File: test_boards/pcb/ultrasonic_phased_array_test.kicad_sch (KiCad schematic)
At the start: 18 parts, among them J1 DF40C-80DP-0.4V, U1 OPA2626, U2 OPA2626, U3 OPA2626, U43 AD7699BCP, U45 SN74LV1T34DBV

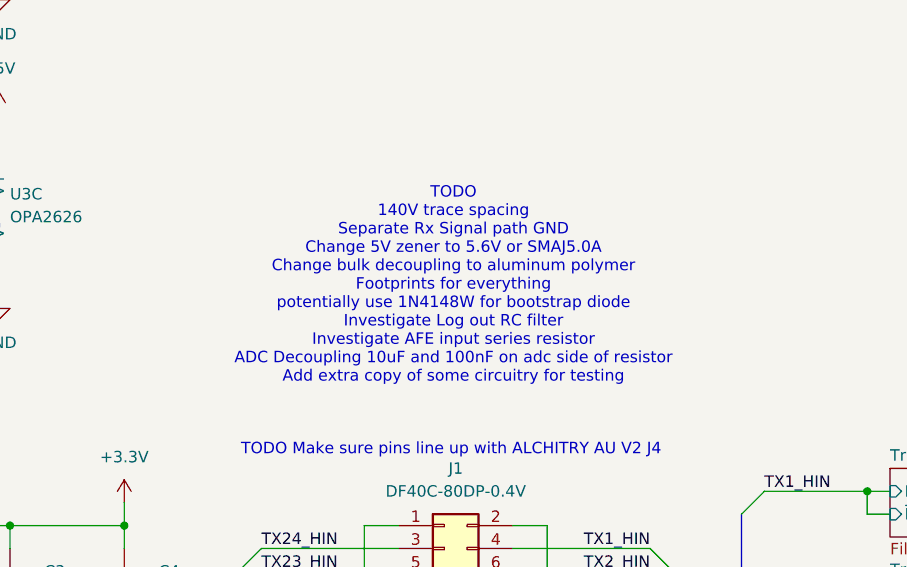
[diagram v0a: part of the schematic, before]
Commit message: w
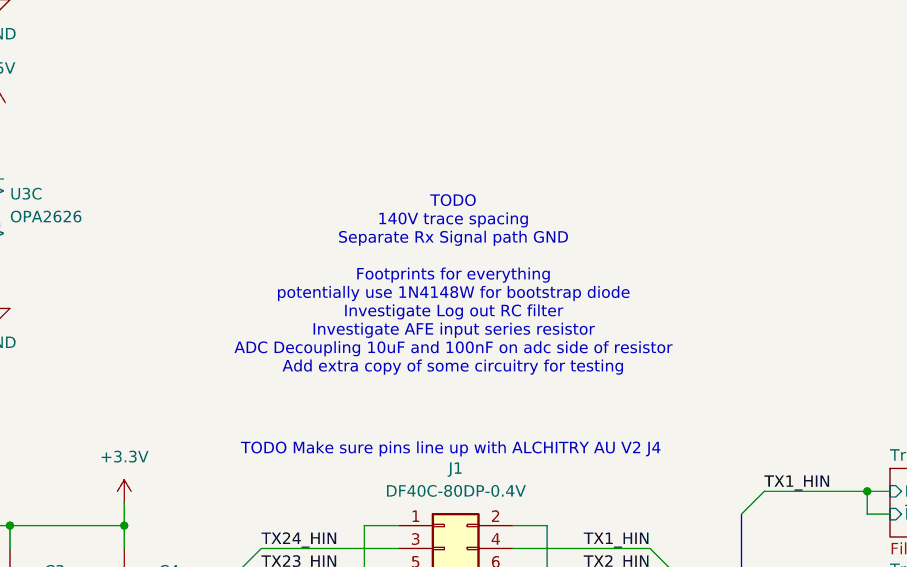
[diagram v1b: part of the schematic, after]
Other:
- note added: "TODO 140V trace spacing Separate Rx Signal path GND Footprints for everything potentially use 1N4148W for bootstrap diode Investigate Log out RC filter Investigate AFE input series resistor ADC Decoupling 10uF and 100nF on adc side of resistor Add extra copy of some circuitry for testing"
- note removed: "TODO 140V trace spacing Separate Rx Signal path GND Change 5V zener to 5.6V or SMAJ5.0A Change bulk decoupling to aluminum polymer Footprints for everything potentially use 1N4148W for bootstrap diode Investigate Log out RC filter Investigate AFE input series resistor ADC Decoupling 10uF and 100nF on adc side of resistor Add extra copy of some circuitry for testing"
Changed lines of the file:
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@@
 		)
 	)
-	(text "TODO\n140V trace spacing\nSeparate Rx Signal path GND\nChange 5V zener to 5.6V or SMAJ5.0A\nChange bulk decoupling to aluminum polymer\nFootprints for everything\npotentially use 1N4148W for bootstrap diode\nInvestigate Log out RC filter\nInvestigate AFE input series resistor\nADC Decoupling 10uF and 100nF on adc side of resistor\nAdd extra copy of some circuitry for testing"
+	(text "TODO\n140V trace spacing\nSeparate Rx Signal path GND\n\nFootprints for everything\npotentially use 1N4148W for bootstrap diode\nInvestigate Log out RC filter\nInvestigate AFE input series resistor\nADC Decoupling 10uF and 100nF on adc side of resistor\nAdd extra copy of some circuitry for testing"
 		(exclude_from_sim no)
 		(at 206.756 68.58 0)
